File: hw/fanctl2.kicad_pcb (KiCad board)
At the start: 2 copper layers, 99.1 x 76.2 mm, 77 parts, among them P0 CONN_01X02, P1 MOLEX_PWR, Q0 FAN_PMOS, Q1 FAN_PMOS, Q2 FAN_PMOS, Q3 FAN_PMOS, Q4 FAN_PMOS, Q5 FAN_PMOS, Q6 BC413, U0 F2_ULN2003, U1 7400, Y0 Crystal_Small

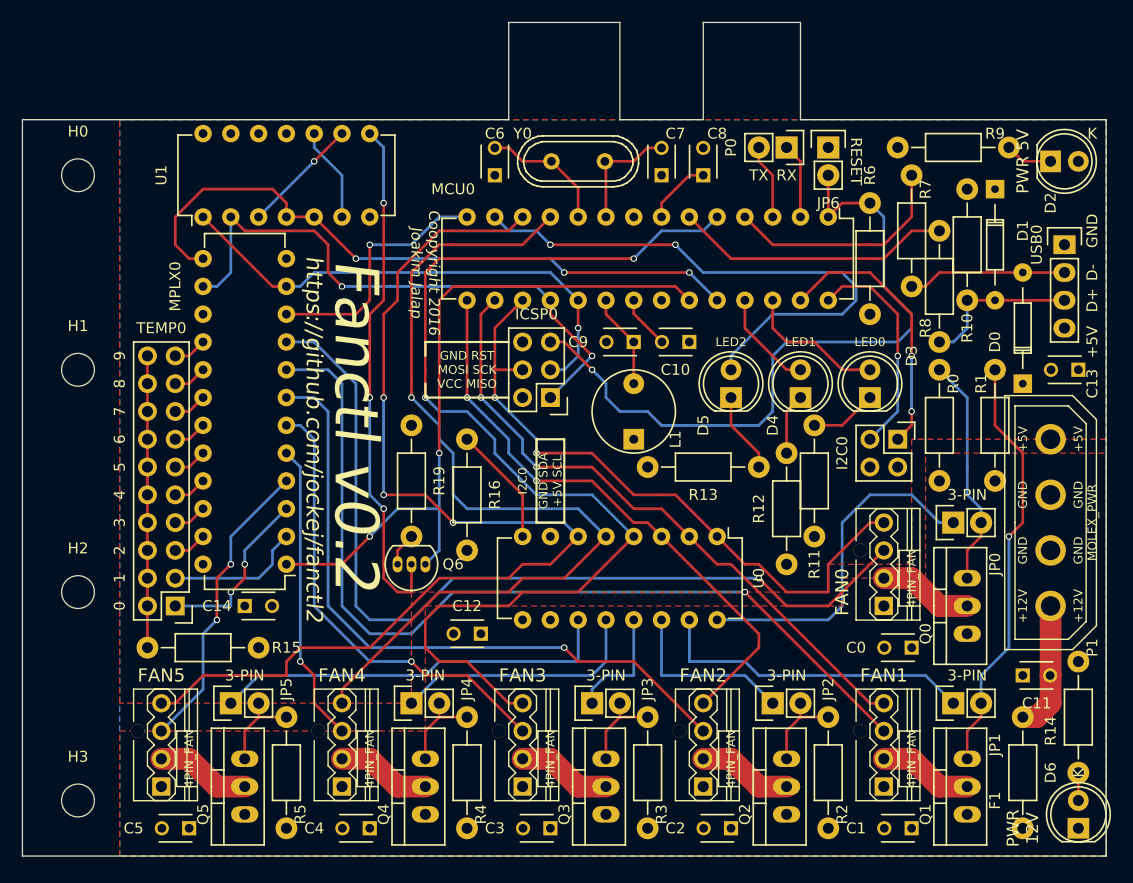
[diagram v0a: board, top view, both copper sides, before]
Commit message: Tons of changes
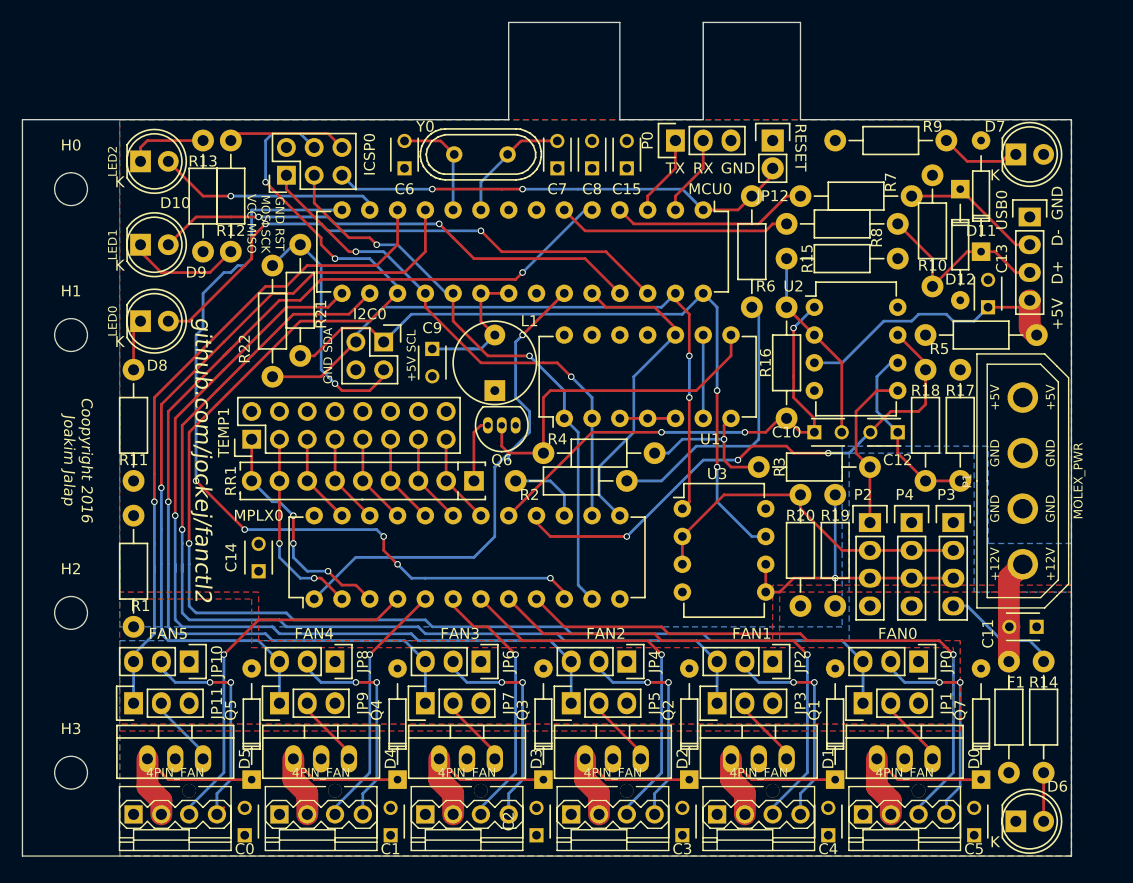
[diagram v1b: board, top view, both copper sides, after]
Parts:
- removed Q0: FAN_PMOS, TO_SOT_Packages_THT:TO-220_Neutral123_Vertical
- removed R0: FANCTL2_R, Resistors_ThroughHole:Resistor_Horizontal_RM10mm
- removed TEMP0: TMP_SNSR_HDR, Pin_Headers:Pin_Header_Straight_2x10
- removed U0: F2_ULN2003, Housings_DIP:DIP-16_W7.62mm
- added C15: 22n, Capacitors_ThroughHole:C_Disc_D3_P2.5, F.Cu at (107.3, 87.0)
- added D10: LED, LEDs:LED-5MM, F.Cu at (62.9, 86.4)
- added D11: ZENER, Diodes_ThroughHole:Diode_DO-35_SOD27_Horizontal_RM10, F.Cu at (139.7, 94.6)
- added D12: ZENER, Diodes_ThroughHole:Diode_DO-35_SOD27_Horizontal_RM10, F.Cu at (137.8, 88.9)
- added D7: LED, LEDs:LED-5MM, F.Cu at (142.9, 85.7)
- added D8: LED, LEDs:LED-5MM, F.Cu at (62.9, 101.0)
- added D9: LED, LEDs:LED-5MM, F.Cu at (62.9, 94.0)
- added JP10: JUMPER3, Pin_Headers:Pin_Header_Straight_1x03, F.Cu at (67.3, 132.1)
- added JP11: JUMPER3, Pin_Headers:Pin_Header_Straight_1x03, F.Cu at (62.2, 135.9)
- added JP12: Jumper_NO_Small, Pin_Headers:Pin_Header_Straight_1x02, F.Cu at (120.7, 84.5)
- added JP7: JUMPER3, Pin_Headers:Pin_Header_Straight_1x03, F.Cu at (88.9, 135.9)
- added JP8: JUMPER3, Pin_Headers:Pin_Header_Straight_1x03, F.Cu at (80.6, 132.1)
- added JP9: JUMPER3, Pin_Headers:Pin_Header_Straight_1x03, F.Cu at (75.6, 135.9)
- added P2: CONN_01X04, Pin_Headers:Pin_Header_Straight_1x04, F.Cu at (129.5, 119.4)
- added P3: CONN_01X04, Pin_Headers:Pin_Header_Straight_1x04, F.Cu at (137.2, 119.4)
- added P4: CONN_01X04, Pin_Headers:Pin_Header_Straight_1x04, F.Cu at (133.3, 119.4)
- added Q7: FAN_NMOS, TO_SOT_Packages_THT:TO-220_Neutral123_Vertical, F.Cu at (132.7, 141.0)
- added R17: FANCTL2_R, Resistors_ThroughHole:Resistor_Horizontal_RM10mm, F.Cu at (137.8, 110.5)
- added R18: FANCTL2_R, Resistors_ThroughHole:Resistor_Horizontal_RM10mm, F.Cu at (134.6, 110.5)
- added R20: FANCTL2_R, Resistors_ThroughHole:Resistor_Horizontal_RM10mm, F.Cu at (123.2, 121.9)
- added R21: FANCTL2_R, Resistors_ThroughHole:Resistor_Horizontal_RM10mm, F.Cu at (77.5, 99.1)
- added R22: FANCTL2_R, Resistors_ThroughHole:Resistor_Horizontal_RM10mm, F.Cu at (74.9, 101.0)
- added RR1: RR8, Housings_SIP:SIP9_Housing, F.Cu at (83.2, 115.6)
- added TEMP1: TMP_SNSR_HDR, Pin_Headers:Pin_Header_Straight_2x08, F.Cu at (73.0, 111.8)
- added U2: LM358, Housings_DIP:DIP-8_W7.62mm, F.Cu at (124.5, 99.7)
- added U3: P82B96, Housings_DIP:DIP-8_W7.62mm, F.Cu at (112.4, 118.1)
- C0, C1, C13, C14, C2, C3, C4, C5, C8, C9: value Decoupler -> 0.1u
- C10, C12: value Decoupler -> C
- C6, C7: value Decoupler -> 22p
- D0, D1: value ZENER -> D
- D2, D3, D4, D5: value LED -> D; footprint LEDs:LED-5MM -> Diodes_ThroughHole:Diode_DO-35_SOD27_Horizontal_RM10
- JP0, JP1, JP2, JP3, JP4, JP5: value Jumper_NC_Small -> JUMPER3; footprint Pin_Headers:Pin_Header_Straight_1x02 -> Pin_Headers:Pin_Header_Straight_1x03
- JP6: value Jumper_NO_Small -> JUMPER3; footprint Pin_Headers:Pin_Header_Straight_1x02 -> Pin_Headers:Pin_Header_Straight_1x03
- L1: value INDUCTOR_SMALL -> 10uH
- P0: value CONN_01X02 -> CONN_01X03; footprint Pin_Headers:Pin_Header_Straight_1x02 -> Pin_Headers:Pin_Header_Straight_1x03
- Q1, Q2, Q3, Q4, Q5: value FAN_PMOS -> FAN_NMOS
- R1, R6: value FANCTL2_R -> 10K
- R16: value R -> FANCTL2_R
- R2, R4: value FANCTL2_R -> 10k
- R3, R5: value FANCTL2_R -> R
- R7, R8: value FANCTL2_R -> 68
- moved R1 79.9 mm to (62.2, 123.8), turned to 270 degrees
- moved R5 75.1 mm to (139.7, 102.2), turned to 0 degrees
- moved C5 71.8 mm to (139.1, 148.0), turned to 90 degrees
- moved R15 68.4 mm to (127.0, 95.2), turned to 0 degrees
- moved D2 65.5 mm to (113.0, 142.9), turned to 90 degrees
- moved C0 63.3 mm to (72.4, 148.0), turned to 90 degrees
- moved R11 62.4 mm to (62.2, 110.5)
- moved R12 58.3 mm to (71.1, 89.5), turned to 270 degrees
- moved JP6 56.7 mm to (94.0, 132.1), turned to 270 degrees
- moved D5 56.0 mm to (73.0, 142.9)
- moved D1 55.9 mm to (126.4, 142.9), turned to 90 degrees
- moved R13 52.0 mm to (68.6, 89.5), turned to 90 degrees
- moved D4 50.8 mm to (86.4, 142.9)
- moved I2C0 47.8 mm to (85.1, 102.9)
- moved C1 47.6 mm to (85.7, 148.0), turned to 90 degrees
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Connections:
- C0 pad 2: GND -> 12VGND
- C1 pad 2: GND -> 12VGND
- C10 pad 1: GND -> I5V
- C11 pad 1: GND -> 12VGND
- C12 pad 1: +12V -> Net-(C12-Pad1)
- C12 pad 2: GND -> I12V
- C13 pad 1: +5V -> Net-(C13-Pad1)
- C2 pad 2: GND -> 12VGND
- C3 pad 2: GND -> 12VGND
- C4 pad 2: GND -> 12VGND
- C5 pad 2: GND -> 12VGND
- D0 pad 1: GND -> Net-(D0-Pad1)
- D0 pad 2: Net-(D0-Pad2) -> 12VGND
- D1 pad 1: GND -> Net-(D1-Pad1)
- D1 pad 2: Net-(D1-Pad2) -> 12VGND
- D2 pad 2: +5V -> 12VGND
- D3 pad 2: LED0 -> 12VGND
- D4 pad 2: LED1 -> 12VGND
- D5 pad 2: LED2 -> 12VGND
- D6 pad 1: GND -> 12VGND
- FAN0 pad 1: GND -> 12VGND
- FAN0 pad 2: Net-(FAN0-Pad2) -> Net-(D0-Pad1)
- FAN0 pad 4: PWM0 -> Net-(FAN0-Pad4)
- FAN1 pad 1: GND -> 12VGND
- FAN1 pad 2: Net-(FAN1-Pad2) -> Net-(D1-Pad1)
- FAN1 pad 4: PWM1 -> Net-(FAN1-Pad4)
- FAN2 pad 1: GND -> 12VGND
- FAN2 pad 2: Net-(FAN2-Pad2) -> Net-(D2-Pad1)
- FAN2 pad 4: PWM2 -> Net-(FAN2-Pad4)
- FAN3 pad 1: GND -> 12VGND
- FAN3 pad 2: Net-(FAN3-Pad2) -> Net-(D3-Pad1)
- FAN3 pad 4: PWM3 -> Net-(FAN3-Pad4)
- FAN4 pad 1: GND -> 12VGND
- FAN4 pad 2: Net-(FAN4-Pad2) -> Net-(D4-Pad1)
- FAN4 pad 4: PWM4 -> Net-(FAN4-Pad4)
- FAN5 pad 1: GND -> 12VGND
- FAN5 pad 2: Net-(FAN5-Pad2) -> Net-(D5-Pad1)
- FAN5 pad 4: PWM5 -> Net-(FAN5-Pad4)
- I2C0 pad 1: Net-(I2C0-Pad1) -> SCL
- I2C0 pad 3: Net-(I2C0-Pad3) -> SDA
- JP0 pad 1: PWM12_0 -> COM5V
- JP0 pad 2: Net-(JP0-Pad2) -> Net-(FAN0-Pad4)
- JP1 pad 1: PWM12_1 -> PWM0
- JP2 pad 1: PWM12_2 -> COM5V
- JP2 pad 2: Net-(JP2-Pad2) -> Net-(FAN1-Pad4)
- JP3 pad 1: PWM12_3 -> PWM1
- JP4 pad 1: PWM12_4 -> COM5V
- JP4 pad 2: Net-(JP4-Pad2) -> Net-(FAN2-Pad4)
- JP5 pad 1: PWM12_5 -> PWM2
- JP6 pad 1: GND -> COM5V
- JP6 pad 2: Net-(ICSP0-Pad5) -> Net-(FAN3-Pad4)
- MCU0 pad 21: Net-(C10-Pad2) -> Net-(C9-Pad1)
- MCU0 pad 27: Net-(I2C0-Pad1) -> SDA
- MCU0 pad 28: Net-(I2C0-Pad3) -> SCL
- MPLX0 pad 16: Net-(MPLX0-Pad16) -> I12V
- MPLX0 pad 17: Net-(MPLX0-Pad17) -> I5V
- P0 pad 1: Net-(MCU0-Pad2) -> Net-(MCU0-Pad3)
- P0 pad 2: Net-(MCU0-Pad3) -> Net-(MCU0-Pad2)
- Q1 pad 1: +12V -> Net-(D1-Pad1)
- Q1 pad 2: Net-(FAN1-Pad2) -> +12V
- Q1 pad 3: Net-(JP1-Pad2) -> Net-(JP3-Pad2)
- Q2 pad 1: +12V -> Net-(D2-Pad1)
- Q2 pad 2: Net-(FAN2-Pad2) -> +12V
- Q2 pad 3: Net-(JP2-Pad2) -> Net-(JP5-Pad2)
- Q3 pad 1: +12V -> Net-(D3-Pad1)
- Q3 pad 2: Net-(FAN3-Pad2) -> +12V
- Q3 pad 3: Net-(JP3-Pad2) -> Net-(JP7-Pad2)
- Q4 pad 1: +12V -> Net-(D4-Pad1)
- Q4 pad 2: Net-(FAN4-Pad2) -> +12V
- Q4 pad 3: Net-(JP4-Pad2) -> Net-(JP9-Pad2)
- Q5 pad 1: +12V -> Net-(D5-Pad1)
- Q5 pad 2: Net-(FAN5-Pad2) -> +12V
- Q5 pad 3: Net-(JP5-Pad2) -> Net-(JP11-Pad2)
- Q6 pad 1: SENS0 -> +5V
- R1 pad 1: +12V -> +5V
- R1 pad 2: Net-(JP1-Pad2) -> COM5V
- R10 pad 1: Net-(D1-Pad2) -> Net-(D11-Pad1)
- R11 pad 2: Net-(D3-Pad1) -> Net-(D8-Pad1)
- R12 pad 2: Net-(D4-Pad1) -> Net-(D9-Pad1)
- R13 pad 2: Net-(D5-Pad1) -> Net-(D10-Pad1)
- R15 pad 1: +5V -> Net-(C10-Pad2)
- R15 pad 2: Net-(R15-Pad2) -> +5V
- R16 pad 1: Net-(R16-Pad1) -> I5V
- R16 pad 2: GND -> Net-(C10-Pad2)
- R19 pad 1: Net-(Q6-Pad3) -> Net-(P2-Pad3)
- R19 pad 2: GND -> +12V
- R2 pad 1: +12V -> +5V
- R2 pad 2: Net-(JP2-Pad2) -> Net-(MPLX0-Pad15)
- R3 pad 1: +12V -> GND
- R3 pad 2: Net-(JP3-Pad2) -> 12VGND
- R4 pad 1: +12V -> GND
- R4 pad 2: Net-(JP4-Pad2) -> Net-(Q6-Pad2)
- R5 pad 1: +12V -> +5V
- R5 pad 2: Net-(JP5-Pad2) -> Net-(C13-Pad1)
- R7 pad 1: Net-(D0-Pad2) -> Net-(D12-Pad1)
- R8 pad 1: Net-(D1-Pad2) -> Net-(D11-Pad1)
- R9 pad 1: Net-(D2-Pad1) -> Net-(D7-Pad1)
- U1 pad 10: Net-(U1-Pad10) -> SEL3
- U1 pad 14: +5V -> VCC
- U1 pad 4: SEL3 -> Net-(U1-Pad3)
- U1 pad 5: SEL3 -> Net-(U1-Pad3)
- U1 pad 6: Net-(U1-Pad10) -> Net-(U1-Pad6)
- U1 pad 9: Net-(U1-Pad3) -> Net-(U1-Pad6)
- USB0 pad 2: Net-(D0-Pad2) -> Net-(D12-Pad1)
- USB0 pad 3: Net-(D1-Pad2) -> Net-(D11-Pad1)
- USB0 pad 4: +5V -> Net-(C13-Pad1)
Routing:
- net PWM0: track 60.3 -> 133.8 mm, vias 2 -> 3
- net SCL: track 0.00 -> 65.6 mm, vias 0 -> 2
- net SDA: track 0.00 -> 60.8 mm, vias 0 -> 2
- net SEL0: track 23.2 -> 75.1 mm, vias 1 -> 5
- net I12V: track 0.00 -> 49.7 mm, vias 0 -> 3
- net I5V: track 0.00 -> 45.2 mm, vias 0 -> 3
- net +5V: track 6.13 -> 49.2 mm, vias 0 -> 1
- net PWM5: track 98.9 -> 60.4 mm, vias 3 -> 1
- net LED0: track 13.0 -> 51.2 mm, vias 0 -> 2
- net TACH1: track 83.3 -> 45.3 mm
- net LED1: track 9.20 -> 46.5 mm, vias 0 -> 2
- net PWM12_5: track 37.1 -> 0.00 mm
- net PWM1: track 58.6 -> 94.5 mm, vias 2 -> 1
- net Net-(JP1-Pad2): track 38.7 -> 6.66 mm, vias 1 -> 0
- net PWM12_0: track 31.8 -> 0.00 mm
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- added copper zone on B.Cu, net 12VGND
- added copper zone on F.Cu, net COM5V
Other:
- board size 99.1 x 76.2 mm -> 95.9 x 76.2 mm
- board text added: "+5V SCL"
- board text added: "GND SDA"
- board text added: "github.com/jockej/fanctl2"
- board text removed: "0"
- board text removed: "1"
- board text removed: "2"
- board text removed: "3"
- board text removed: "3-PIN"
- board text removed: "4"
- board text removed: "5"
- board text removed: "6"
- board text removed: "7"
- board text removed: "8"
- board text removed: "9"
- board text removed: "Fanctl v0.2"
- board text removed: "GND SDA +5V SCL"
- board text removed: "I2C0"
- board text removed: "PWR 12V"
- board text removed: "PWR 5V"
- board text removed: "https://github.com/jockej/fanctl2"
